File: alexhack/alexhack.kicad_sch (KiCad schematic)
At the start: 14 parts, among them J1 ultra, J2 battery, U1 ESP32_NODEMCU, U2 LM7805_TO220

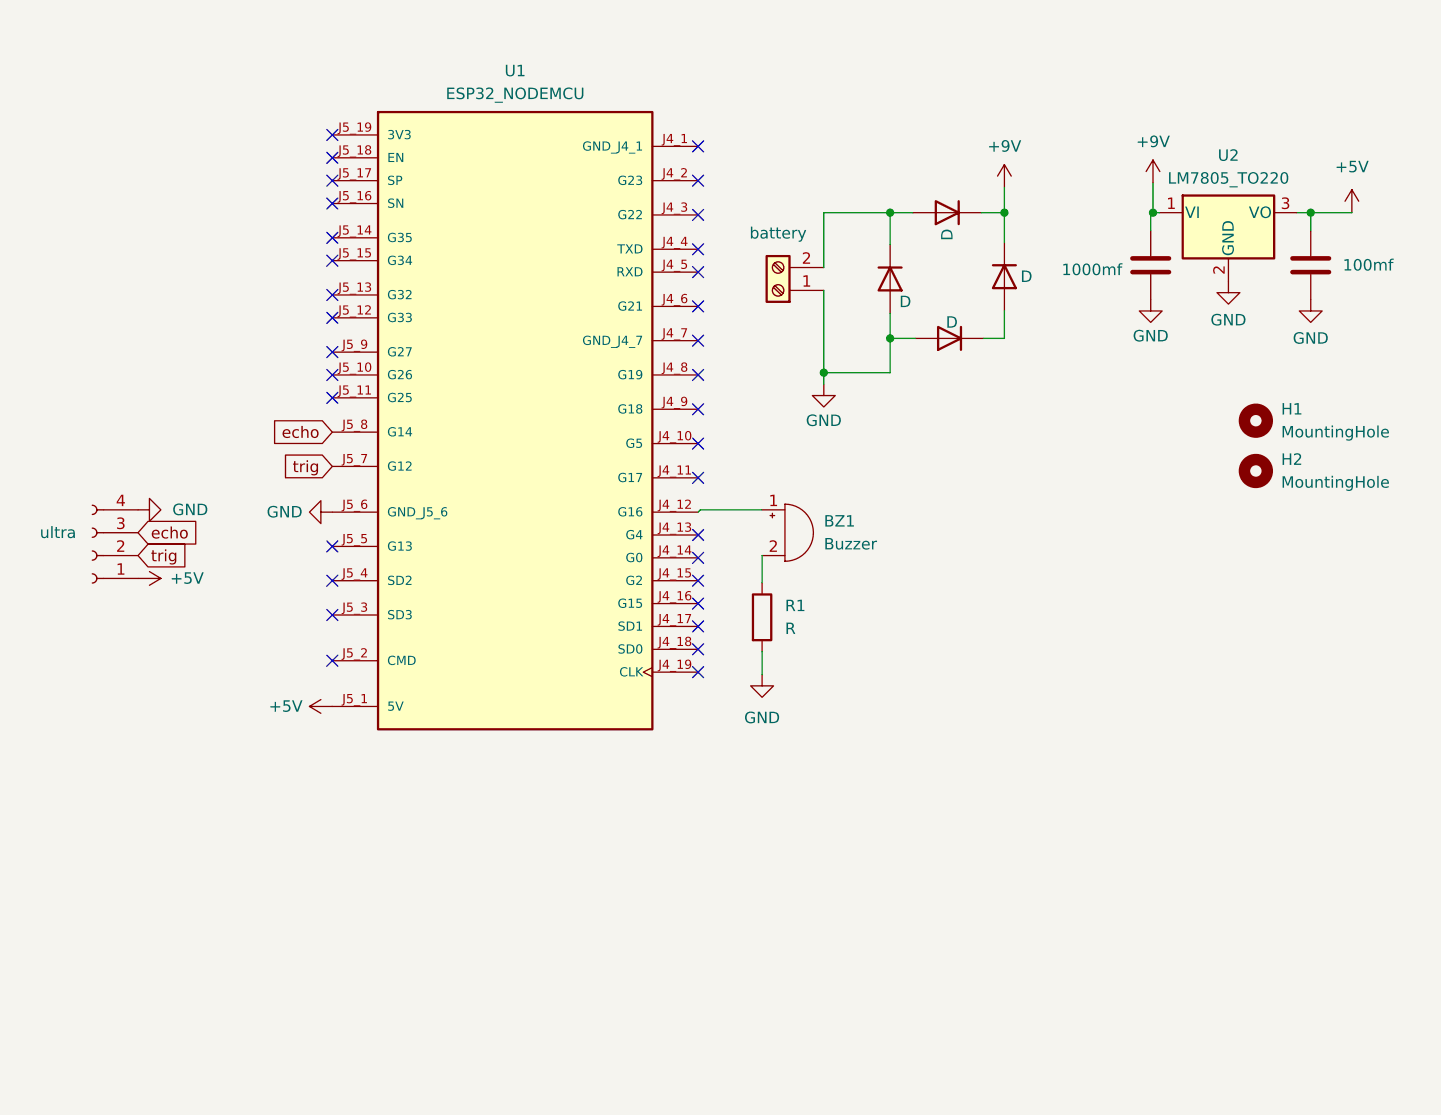
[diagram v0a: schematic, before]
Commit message: Demo
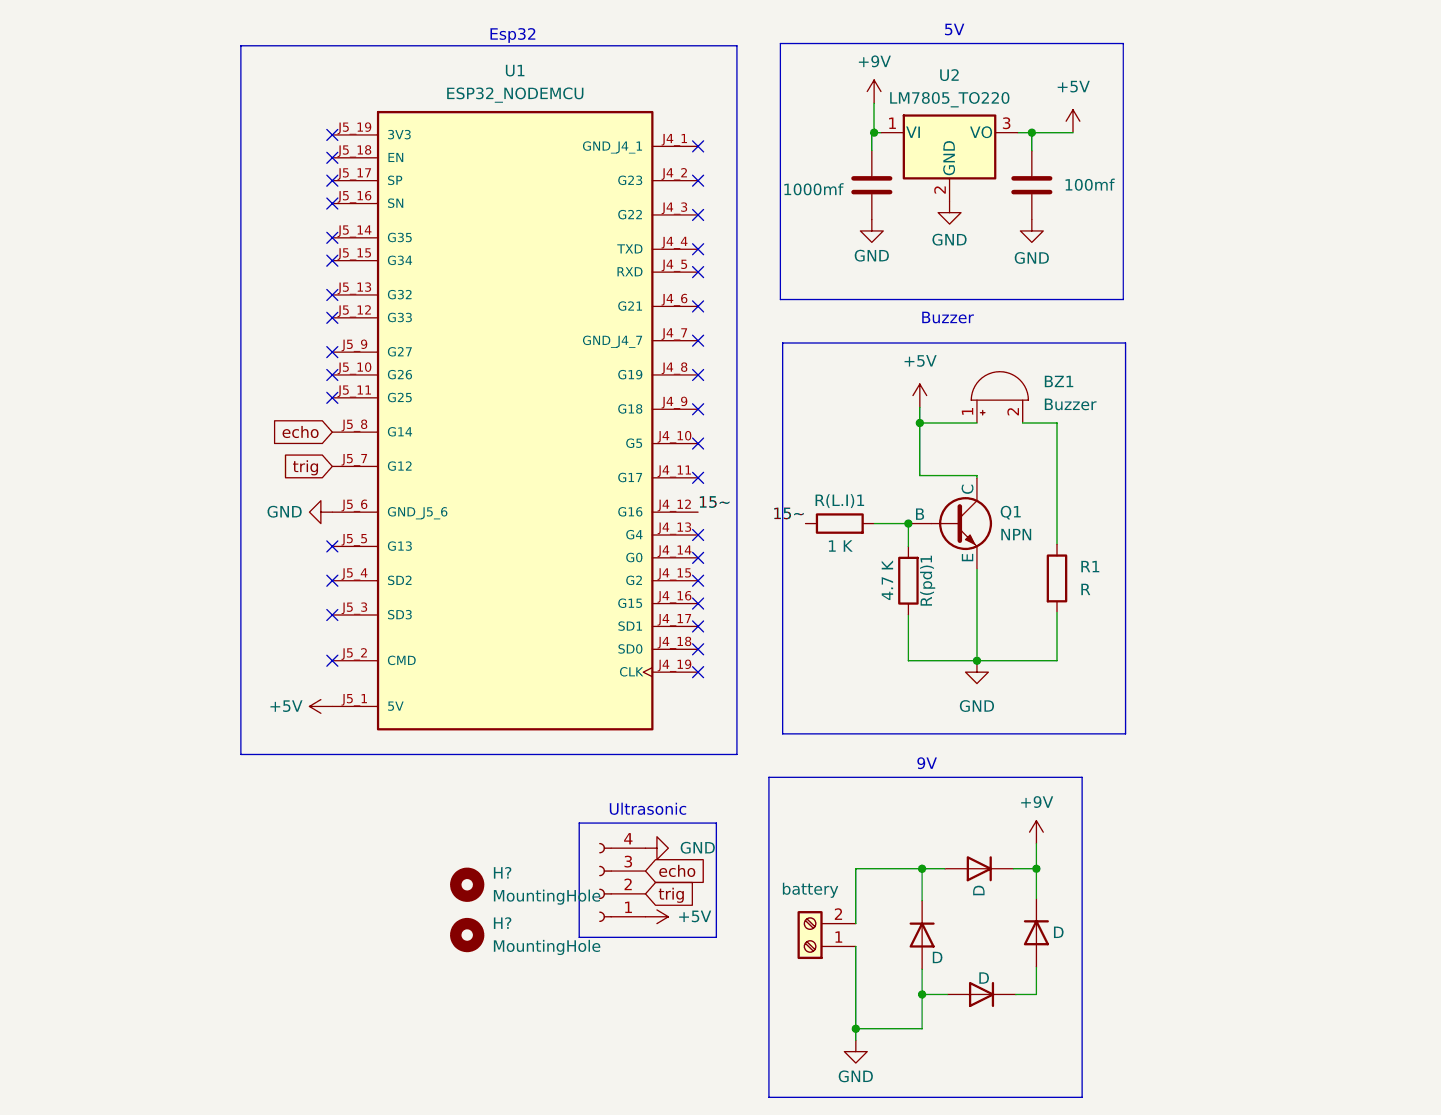
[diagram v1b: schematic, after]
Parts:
- removed H1, H2: MountingHole, MountingHole:MountingHole_2.5mm, symbol Mechanical:MountingHole
- added H? (x2): MountingHole, MountingHole:MountingHole_2.5mm, symbol Mechanical:MountingHole
- added Q1: NPN, B3B-XH-A_LF__SN_:JST_B3B-XH-A_LF__SN_, symbol Simulation_SPICE:NPN
- added R(L.I)1: 1 K, Resistor_THT:R_Axial_DIN0204_L3.6mm_D1.6mm_P5.08mm_Horizontal, symbol Device:R
- added R(pd)1: 4.7 K, Resistor_THT:R_Axial_DIN0204_L3.6mm_D1.6mm_P5.08mm_Horizontal, symbol Device:R
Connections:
- net +5V: now also BZ1.1 (+), Q1.1 (C)
- net GND: now also Q1.3 (E), R(pd)1.1
- net 15~: now reaches U1.J4_12 (G16)
- net 15~: now also R(L.I)1.1; no longer BZ1.1 (+)
- new net: Q1.2 (B), R(L.I)1.2, R(pd)1.2
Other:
- note added: "5V"
- note added: "9V"
- note added: "Buzzer"
- note added: "Esp32"
- note added: "Ultrasonic"
- moved on the sheet: R1, U2
